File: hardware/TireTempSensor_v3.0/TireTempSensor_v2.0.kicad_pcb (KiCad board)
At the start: 4 copper layers, 75.7 x 20 mm, 75 parts, among them IC2 MLX90621ESF-BAB-000-SP, IC4 TPS54202HDDCR, J2 Main connector, J3 FTSH-107-01-L-D-K, T10 TP_+5V, T14 TP_+3.3V, T15 TP_+2.6V, U1 STM32G0C1KCTxN, U2 MIC5306-2.6YD5-TR, U3 NCP715SQ33T2G, U7 ADM3057ExRW, Y1 ATX-11-F-32.000MHZ-F05-T

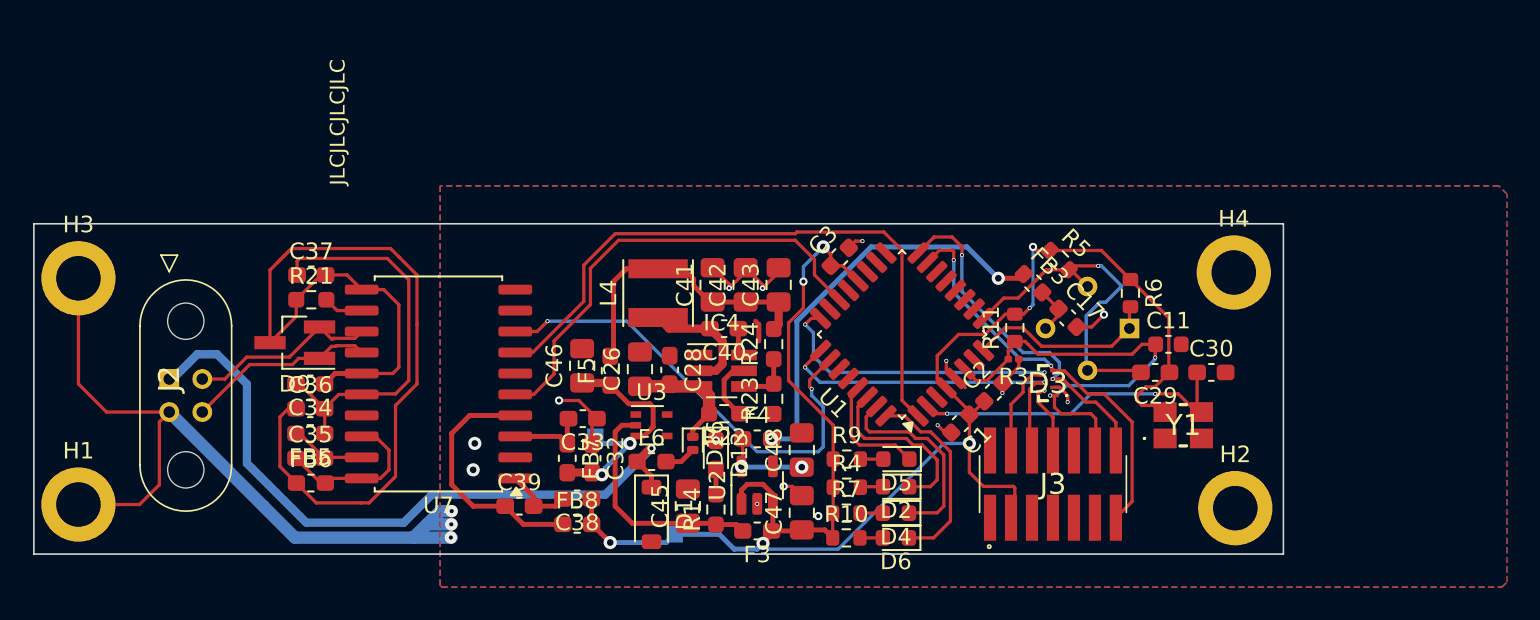
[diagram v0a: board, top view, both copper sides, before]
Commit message: Gotowe do sprawdzenia
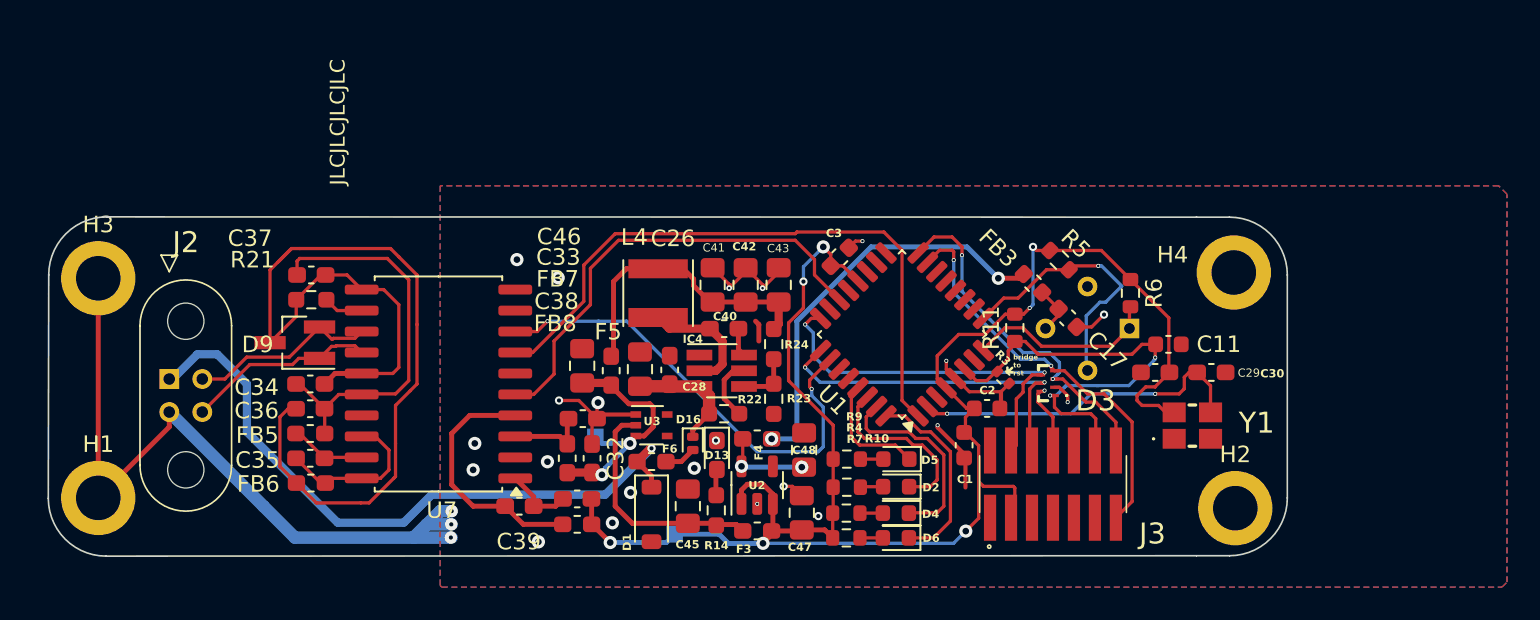
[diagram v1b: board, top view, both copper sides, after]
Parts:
- R3: footprint Resistor_SMD:R_0201_0603Metric -> Resistor_SMD:R_0402_1005Metric
- moved C1 1.33 mm to (150.9, 102.8), turned to -90 degrees
- moved R3 1.27 mm to (153.3, 98.7), turned to 135 degrees
- moved H1 1.26 mm to (98.5, 106.0)
- moved H3 1.20 mm to (98.5, 92.7)
- moved C2 1.05 mm to (152.3, 100.6), turned to 0 degrees
- moved Y1 0.55 mm to (164.8, 101.6)
- moved C48 0.14 mm to (141.2, 103.1)
- moved F5 0.06 mm to (129.6, 98.3)
- moved D13 0.06 mm to (136.0, 103.4)
- moved R14 0.05 mm to (135.9, 106.8)
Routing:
- net GND: track 79.4 -> 82.8 mm, vias 18 -> 25
- net /SDA: track 18.0 -> 16.5 mm
- net +24V: track 41.8 -> 40.7 mm
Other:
- board size 75.7 x 20 mm -> 75 x 20.5 mm
- board text added: "bridge to rst"
